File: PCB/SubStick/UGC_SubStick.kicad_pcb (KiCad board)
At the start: 2 copper layers, 50.4 x 31.6 mm, 1 part, among them SW1 GL18_SW

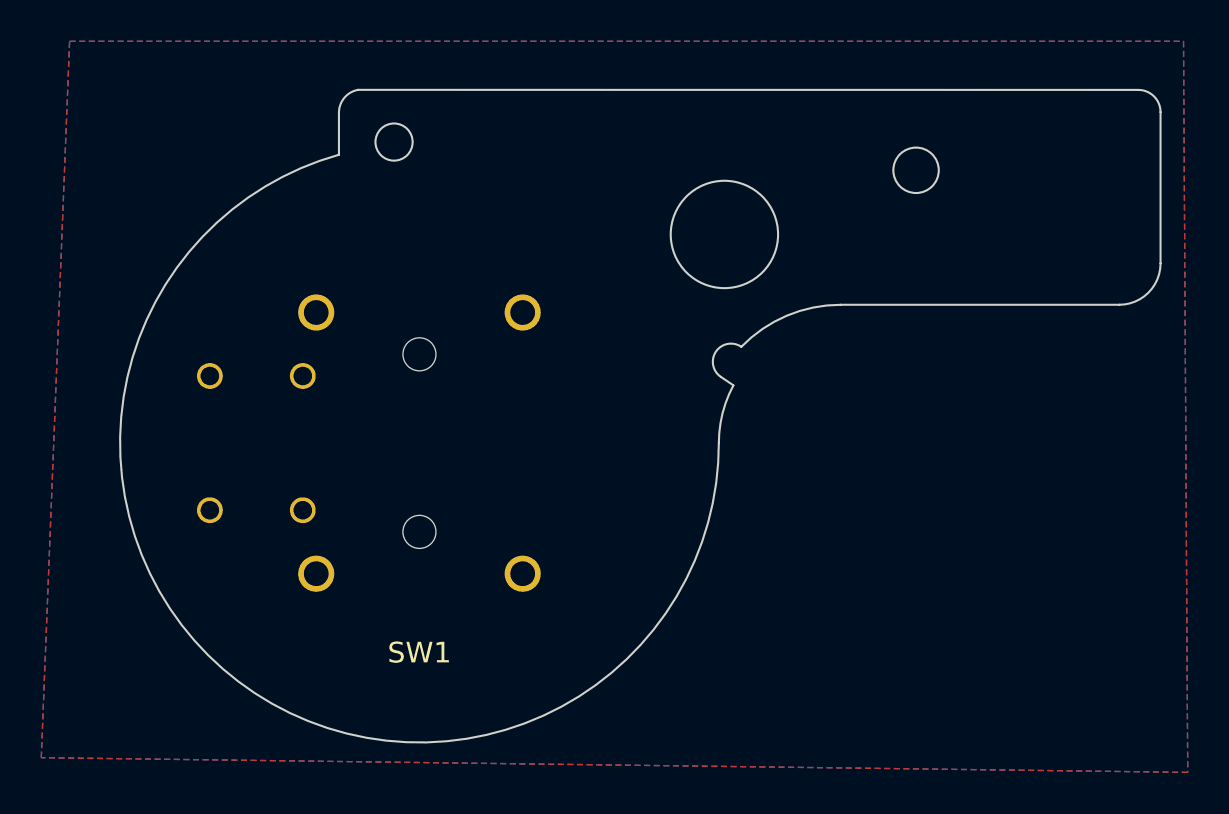
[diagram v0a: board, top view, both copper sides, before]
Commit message: Update shell and PCB
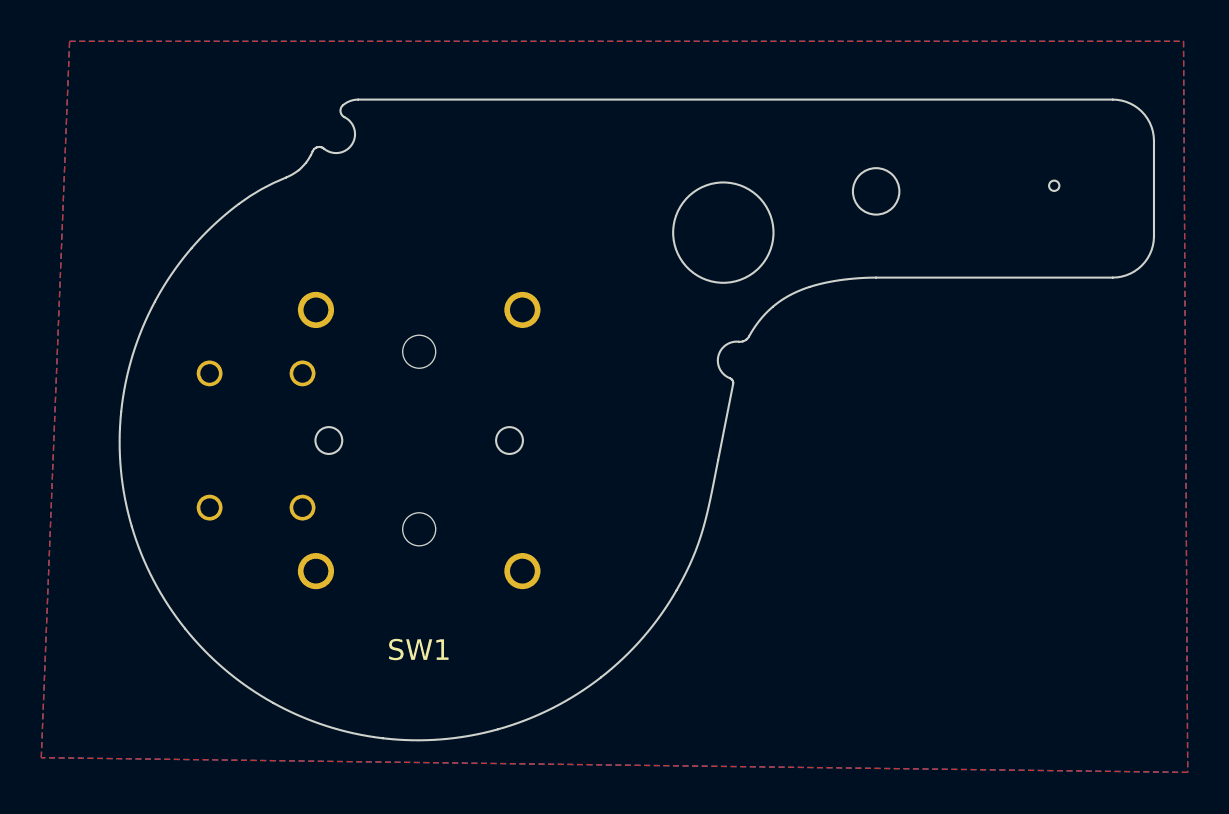
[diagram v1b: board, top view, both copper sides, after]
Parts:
- moved SW1 0.13 mm to (247.2, 149.7)
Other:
- board size 50.4 x 31.6 mm -> 50.1 x 31 mm
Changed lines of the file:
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@@
   (net 4 "unconnected-(SW1-4-PadS4)")
   (footprint "hhl:GL18" (layer "F.Cu")
-    (at 247.220512 149.813671)
+    (at 247.2072 149.688518)
     (property "MPN" "GL18")
     (property "Sheetfile" "UGC_SubStick.kicad_sch")
@@
       (net 4 "unconnected-(SW1-4-PadS4)") (pinfunction "4") (pintype "input"))
   )
-  (gr_arc (start 261.720773 149.81334) (mid 238.453936 161.363767) (end 243.320772 135.847656)
+  (gr_curve (pts (xy 236.182716 140.373821) (xy 235.498868 141.170014) (xy 234.903887 142.038443) (xy 234.408371 142.963672))
     (stroke (width 0.1) (type solid)) (layer "Edge.Cuts"))
-  (gr_line (start 243.320766 133.81334) (end 243.320772 135.847656)
+  (gr_curve (pts (xy 262.416512 146.875826) (xy 262.419466 146.901486) (xy 262.418425 146.927449) (xy 262.413427 146.952791))
     (stroke (width 0.1) (type solid)) (layer "Edge.Cuts"))
-  (gr_line (start 283.11303 141.113576) (end 283.11303 133.780606)
+  (gr_curve (pts (xy 264.33381 143.213824) (xy 264.840979 142.782004) (xy 265.432345 142.469536) (xy 266.125889 142.247344))
     (stroke (width 0.1) (type solid)) (layer "Edge.Cuts"))
-  (gr_circle (center 245.989918 135.233341) (end 245.089918 135.233341)
+  (gr_arc (start 243.517695 133.447452) (mid 243.86174 133.246104) (end 244.25418 133.176111)
+    (stroke (width 0.1) (type solid)) (layer "Edge.Cuts"))
+  (gr_curve (pts (xy 261.687781 150.631904) (xy 261.929663 149.405533) (xy 262.171545 148.179162) (xy 262.413427 146.952791))
+    (stroke (width 0.1) (type solid)) (layer "Edge.Cuts"))
+  (gr_curve (pts (xy 262.396021 146.801576) (xy 262.406646 146.825118) (xy 262.413559 146.850166) (xy 262.416512 146.875826))
+    (stroke (width 0.1) (type solid)) (layer "Edge.Cuts"))
+  (gr_curve (pts (xy 233.286784 153.849988) (xy 233.8177 155.652394) (xy 234.69568 157.33392) (xy 235.871146 158.800026))
+    (stroke (width 0.1) (type solid)) (layer "Edge.Cuts"))
+  (gr_arc (start 262.258094 146.671154) (mid 261.69711 145.598301) (end 262.689001 144.904134)
+    (stroke (width 0.1) (type solid)) (layer "Edge.Cuts"))
+  (gr_curve (pts (xy 245.457574 164.109906) (xy 247.323163 164.328607) (xy 249.213601 164.181329) (xy 251.022835 163.676242))
+    (stroke (width 0.1) (type solid)) (layer "Edge.Cuts"))
+  (gr_curve (pts (xy 240.14013 162.398991) (xy 241.784364 163.309899) (xy 243.590696 163.891054) (xy 245.457574 164.109906))
+    (stroke (width 0.1) (type solid)) (layer "Edge.Cuts"))
+  (gr_arc (start 243.589841 134.027633) (mid 243.951806 135.351149) (end 242.594525 135.552392)
+    (stroke (width 0.1) (type solid)) (layer "Edge.Cuts"))
+  (gr_curve (pts (xy 266.125889 142.247344) (xy 267.437638 141.827097) (xy 268.899751 141.798227) (xy 269.339269 141.798227))
+    (stroke (width 0.1) (type solid)) (layer "Edge.Cuts"))
+  (gr_curve (pts (xy 242.123835 135.571284) (xy 242.156289 135.539286) (xy 242.194682 135.513934) (xy 242.236854 135.496653))
+    (stroke (width 0.1) (type solid)) (layer "Edge.Cuts"))
+  (gr_curve (pts (xy 242.04761 135.683234) (xy 242.065487 135.641311) (xy 242.091381 135.603281) (xy 242.123835 135.571284))
+    (stroke (width 0.1) (type solid)) (layer "Edge.Cuts"))
+  (gr_curve (pts (xy 232.774982 148.296871) (xy 232.582661 150.163609) (xy 232.756548 152.049892) (xy 233.286784 153.849988))
+    (stroke (width 0.1) (type solid)) (layer "Edge.Cuts"))
+  (gr_circle (center 251.5822 149.688518) (end 250.9322 149.688518)
     (stroke (width 0.1) (type solid)) (fill none) (layer "Edge.Cuts"))
-  (gr_arc (start 283.11303 141.113576) (mid 282.527272 142.527762) (end 281.11311 143.113576)
+  (gr_curve (pts (xy 234.408371 142.963672) (xy 233.522291 144.618165) (xy 232.967327 146.429893) (xy 232.774982 148.296871))
     (stroke (width 0.1) (type solid)) (layer "Edge.Cuts"))
-  (gr_line (start 267.620701 143.114115) (end 281.11311 143.113576)
+  (gr_arc (start 238.47358 138.230022) (mid 239.5728 137.5156) (end 240.757606 136.954424)
     (stroke (width 0.1) (type solid)) (layer "Edge.Cuts"))
-  (gr_arc (start 261.720773 149.81334) (mid 261.899934 148.371175) (end 262.426171 147.016548)
+  (gr_curve (pts (xy 262.339918 146.722765) (xy 262.363571 146.745131) (xy 262.38263 146.771904) (xy 262.396021 146.801576))
     (stroke (width 0.1) (type solid)) (layer "Edge.Cuts"))
-  (gr_circle (center 261.989931 139.70834) (end 259.389931 139.70834)
+  (gr_circle (center 242.8322 149.688518) (end 242.1822 149.688518)
     (stroke (width 0.1) (type solid)) (fill none) (layer "Edge.Cuts"))
-  (gr_arc (start 261.817365 146.605903) (mid 261.582331 145.379266) (end 262.810208 145.150792)
+  (gr_curve (pts (xy 238.47358 138.230022) (xy 237.634302 138.859248) (xy 236.866138 139.578124) (xy 236.182716 140.373821))
     (stroke (width 0.1) (type solid)) (layer "Edge.Cuts"))
-  (gr_line (start 262.426171 147.016548) (end 261.817365 146.605903)
+  (gr_line (start 269.339269 141.798227) (end 280.79541 141.798227)
     (stroke (width 0.1) (type solid)) (layer "Edge.Cuts"))
-  (gr_arc (start 243.320766 133.81334) (mid 243.580431 133.093181) (end 244.239931 132.704447)
+  (gr_circle (center 261.937726 139.619733) (end 259.507726 139.619733)
+    (stroke (width 0.1) (type solid)) (fill none) (layer "Edge.Cuts"))
+  (gr_curve (pts (xy 259.6752 156.938683) (xy 260.947044 154.71543) (xy 261.163485 153.290147) (xy 261.687781 150.631904))
     (stroke (width 0.1) (type solid)) (layer "Edge.Cuts"))
-  (gr_circle (center 271.272 136.6012) (end 270.172 136.6012)
+  (gr_arc (start 243.589841 134.027633) (mid 243.397445 133.756981) (end 243.517695 133.447452)
+    (stroke (width 0.1) (type solid)) (layer "Edge.Cuts"))
+  (gr_line (start 280.79541 133.176111) (end 244.25418 133.176111)
+    (stroke (width 0.1) (type solid)) (layer "Edge.Cuts"))
+  (gr_curve (pts (xy 251.022835 163.676242) (xy 252.834993 163.170339) (xy 254.531141 162.315171) (xy 256.015561 161.158883))
+    (stroke (width 0.1) (type solid)) (layer "Edge.Cuts"))
+  (gr_curve (pts (xy 263.180662 144.650874) (xy 263.442841 144.181174) (xy 263.796421 143.671376) (xy 264.33381 143.213824))
+    (stroke (width 0.1) (type solid)) (layer "Edge.Cuts"))
+  (gr_curve (pts (xy 235.871146 158.800026) (xy 237.046357 160.265812) (xy 238.496527 161.488432) (xy 240.14013 162.398991))
+    (stroke (width 0.1) (type solid)) (layer "Edge.Cuts"))
+  (gr_curve (pts (xy 242.04761 135.683234) (xy 242.020787 135.74614) (xy 241.992431 135.806999) (xy 241.962596 135.865913))
+    (stroke (width 0.1) (type solid)) (layer "Edge.Cuts"))
+  (gr_curve (pts (xy 263.055454 144.79838) (xy 263.004514 144.838926) (xy 262.946141 144.869136) (xy 262.88362 144.887307))
+    (stroke (width 0.1) (type solid)) (layer "Edge.Cuts"))
+  (gr_curve (pts (xy 256.015561 161.158883) (xy 257.498301 160.003905) (xy 258.741827 158.570271) (xy 259.6752 156.938683))
+    (stroke (width 0.1) (type solid)) (layer "Edge.Cuts"))
+  (gr_curve (pts (xy 242.236854 135.496653) (xy 242.279026 135.479373) (xy 242.324171 135.470494) (xy 242.369746 135.470518))
+    (stroke (width 0.1) (type solid)) (layer "Edge.Cuts"))
+  (gr_arc (start 280.79541 133.176111) (mid 282.209624 133.761897) (end 282.79541 135.176111)
+    (stroke (width 0.1) (type solid)) (layer "Edge.Cuts"))
+  (gr_arc (start 282.79541 139.798227) (mid 282.209624 141.212441) (end 280.79541 141.798227)
+    (stroke (width 0.1) (type solid)) (layer "Edge.Cuts"))
+  (gr_circle (center 269.339269 137.621378) (end 268.214269 137.621378)
     (stroke (width 0.1) (type solid)) (fill none) (layer "Edge.Cuts"))
-  (gr_arc (start 262.810208 145.150792) (mid 265.008784 143.644311) (end 267.620701 143.114115)
+  (gr_line (start 282.79541 139.798227) (end 282.79541 135.176111)
     (stroke (width 0.1) (type solid)) (layer "Edge.Cuts"))
-  (gr_line (start 282.048648 132.70734) (end 244.239931 132.704447)
+  (gr_circle (center 277.963716 137.350698) (end 277.713716 137.350698)
+    (stroke (width 0.1) (type solid)) (fill none) (layer "Edge.Cuts"))
+  (gr_curve (pts (xy 263.180662 144.650874) (xy 263.148929 144.707724) (xy 263.106395 144.757833) (xy 263.055454 144.79838))
     (stroke (width 0.1) (type solid)) (layer "Edge.Cuts"))
-  (gr_arc (start 282.048648 132.70734) (mid 282.801814 133.024827) (end 283.11303 133.780606)
+  (gr_curve (pts (xy 241.379633 136.594202) (xy 241.133714 136.769246) (xy 241.046288 136.822058) (xy 240.757606 136.954424))
+    (stroke (width 0.1) (type solid)) (layer "Edge.Cuts"))
+  (gr_curve (pts (xy 242.369746 135.470518) (xy 242.41054 135.47054) (xy 242.451017 135.477693) (xy 242.489348 135.491654))
+    (stroke (width 0.1) (type solid)) (layer "Edge.Cuts"))
+  (gr_curve (pts (xy 241.962596 135.865913) (xy 241.845174 136.068866) (xy 241.78793 136.154711) (xy 241.72709 136.236165))
+    (stroke (width 0.1) (type solid)) (layer "Edge.Cuts"))
+  (gr_curve (pts (xy 262.258094 146.671154) (xy 262.288468 146.682866) (xy 262.316264 146.700398) (xy 262.339918 146.722765))
+    (stroke (width 0.1) (type solid)) (layer "Edge.Cuts"))
+  (gr_curve (pts (xy 242.489348 135.491654) (xy 242.527678 135.505616) (xy 242.563274 135.526171) (xy 242.594525 135.552392))
+    (stroke (width 0.1) (type solid)) (layer "Edge.Cuts"))
+  (gr_curve (pts (xy 241.72709 136.236165) (xy 241.526644 136.459897) (xy 241.45499 136.529043) (xy 241.379633 136.594202))
+    (stroke (width 0.1) (type solid)) (layer "Edge.Cuts"))
+  (gr_curve (pts (xy 262.88362 144.887307) (xy 262.820486 144.905657) (xy 262.754348 144.911375) (xy 262.689001 144.904134))
     (stroke (width 0.1) (type solid)) (layer "Edge.Cuts"))
   (zone (net 0) (net_name "") (layers "F&B.Cu") (hatch edge 0.5)
